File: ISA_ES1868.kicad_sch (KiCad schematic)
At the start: 119 parts, among them J1 LINE IN, J10 Vol. Btns, J11 ISA BUS, J2 LINE OUT, J3 Joystick/MIDI, J5 Wavetable, J7 SPKR OUT, J8 MIC IN, J9 AUX_A, U1 L78L05, U2 74LS138, U3 ES1868F, U4 93LC66, U7 LM1877, Y1 14.318Mhz

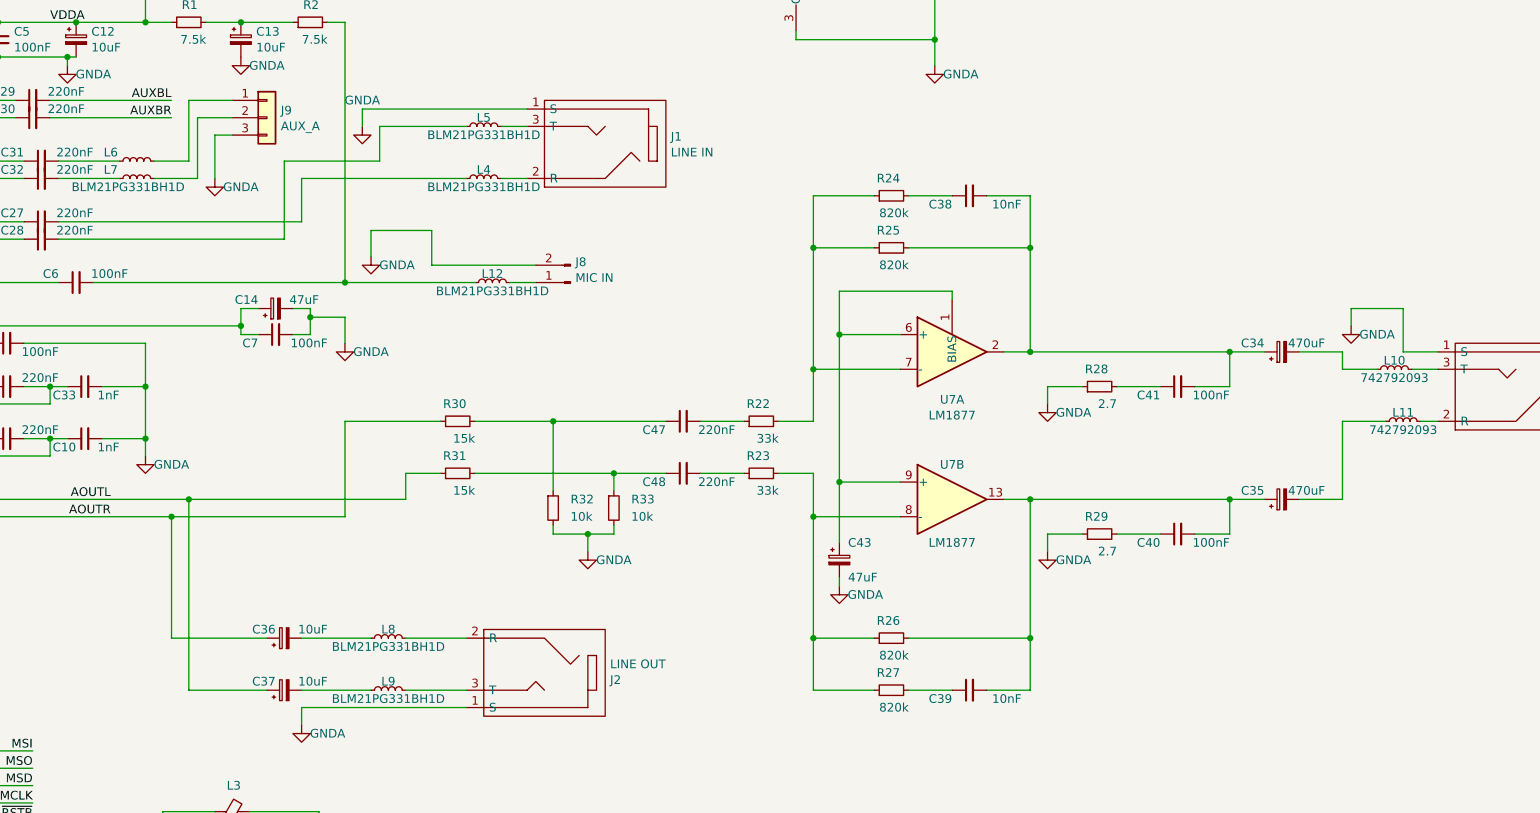
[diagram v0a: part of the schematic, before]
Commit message: Initial import to KiCad 7
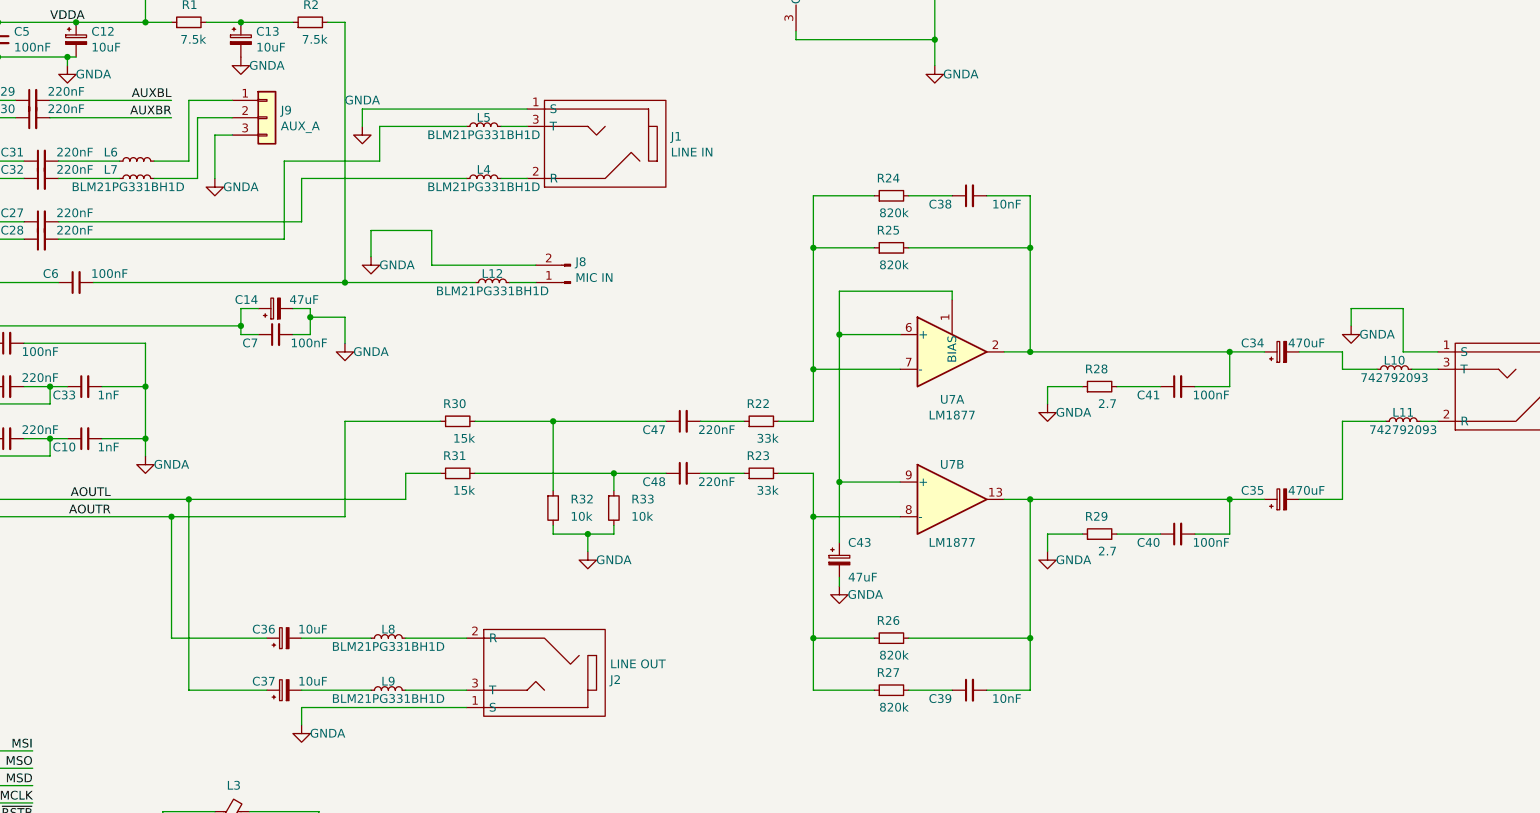
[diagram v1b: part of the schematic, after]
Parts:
- C12, C13, C14, C34, C35, C36, C37, C42, C43, C50, C51, C52: symbol Device:CP_Small -> Device:C_Polarized_Small
- J1, J2, J7: symbol my_components:JACK_TRS_3PINS -> ISA_ES1868-rescue:JACK_TRS_3PINS-my_components
- J3: symbol Connector:DB15_Female_MountingHoles -> Connector:DA15_Receptacle_MountingHoles
- J8: symbol Connector:Conn_01x02_Male -> Connector:Conn_01x02_Pin
- JP3, JP4, JP5, JP6: symbol Device:Jumper_NO_Small -> ISA_ES1868-rescue:Jumper_NO_Small-Device
- L1, L2, L3: symbol Device:Ferrite_Bead_Small -> Device:FerriteBead_Small
